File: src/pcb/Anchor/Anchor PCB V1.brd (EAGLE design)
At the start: 100.1 x 68.7 mm, 89 parts, among them IC1 ENC28J60-I_SS, IC2 TPS23750PWP, IC3 MIC5219-3.3YM5-TR, IC4 DWM1000, J1 0826-1X1T-GJ-F, J2 105017-0001, Q1 32 MHz, Q2 SUD06N10-225L, U1 ATSAMD21G-A, Y1 25 MHz

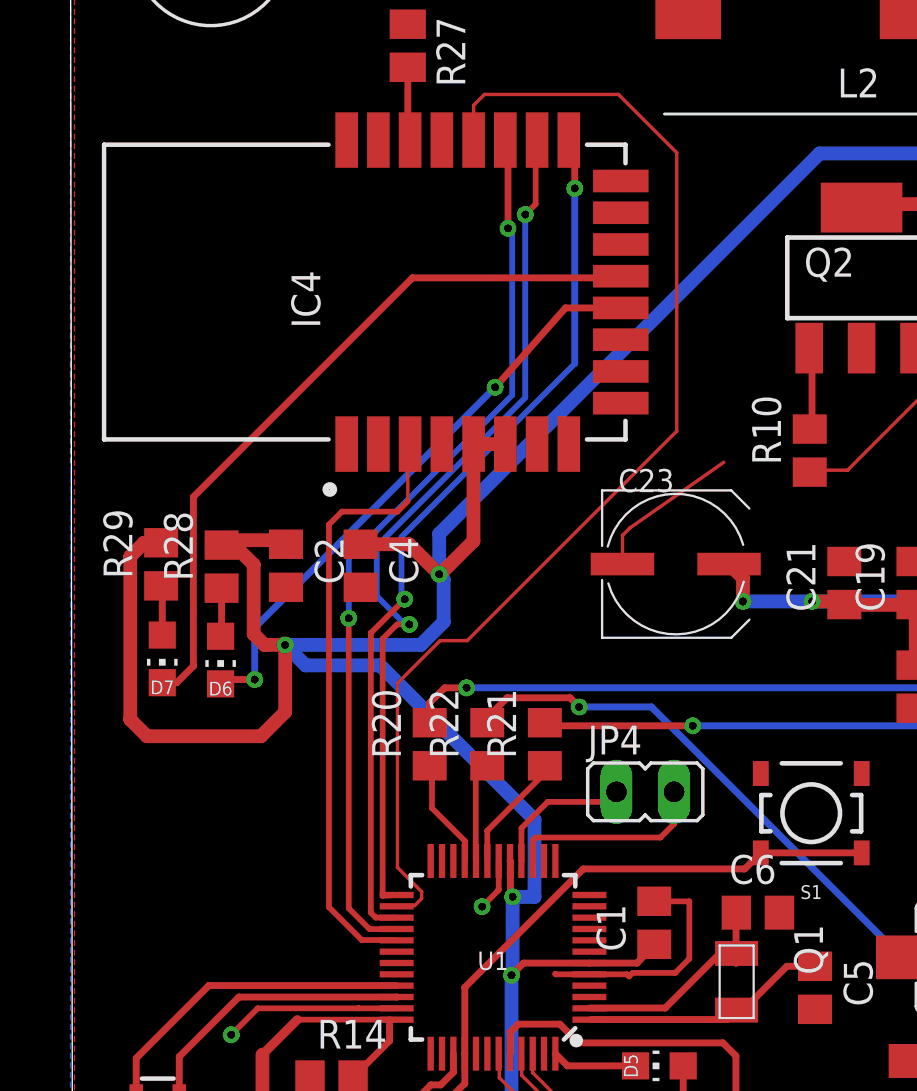
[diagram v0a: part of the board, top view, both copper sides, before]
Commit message: Solving connection problems
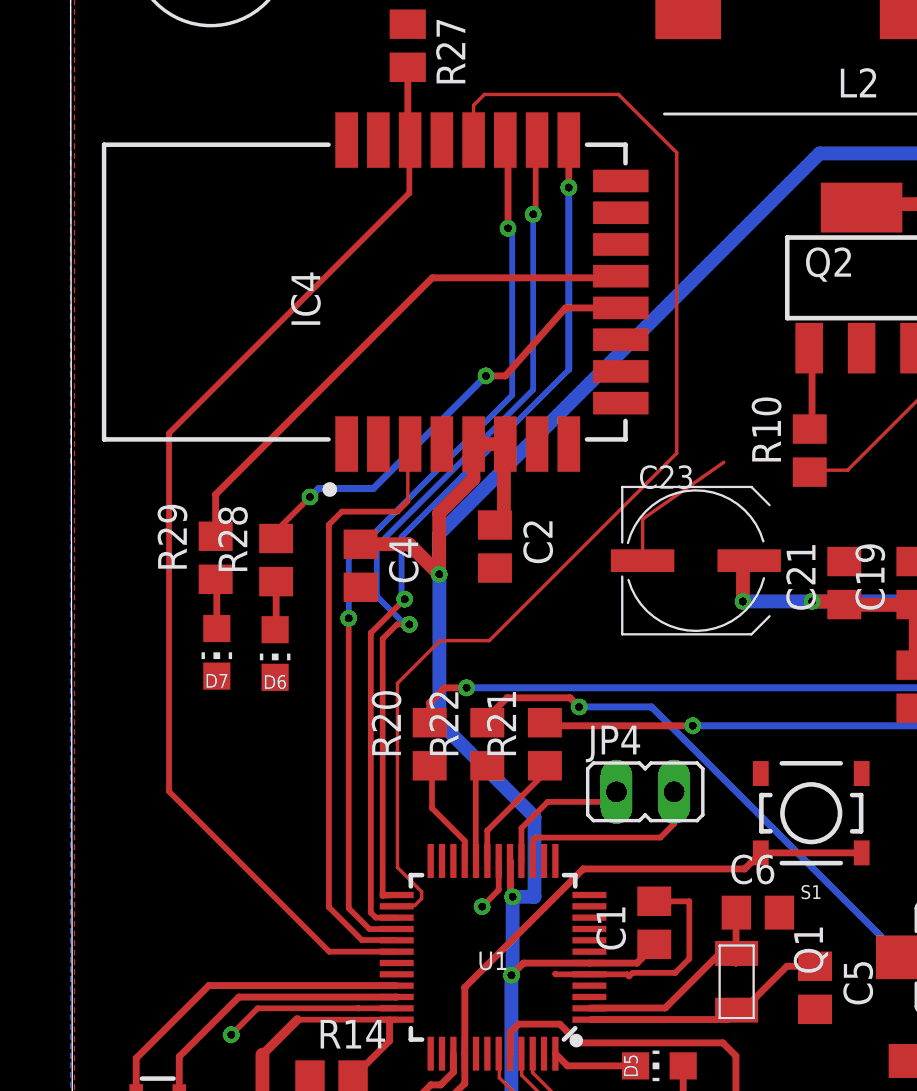
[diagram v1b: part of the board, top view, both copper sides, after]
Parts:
- moved C2 9.25 mm to (18.6, 36.4)
- moved D7 2.42 mm to (6.36, 31.7)
- moved R29 2.42 mm to (6.31, 35.9)
- moved D6 2.42 mm to (8.93, 31.7)
- moved R28 2.42 mm to (8.97, 35.8)
- moved C23 0.90 mm to (27.5, 35.8)
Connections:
- net MISO2_MC renamed MISO2_DWM
- net MOSI2_MC renamed MOSI2_DWM
- net SCK2_MC renamed SCK2_DWM
- net GND: now also D6.C, D7.C
- net IRQ: now also U1.30
- net RXLED_DWM: now also R29.2; no longer D7.C
- net TXLED_DWM: now also R28.2; no longer D6.C
- net VCC: no longer R28.2, R29.2
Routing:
- net IRQ: track 3.25 -> 49.4 mm
- net VCC: track 355.5 -> 319.0 mm, vias 5 -> 4
- net RXLED_DWM: track 32.0 -> 23.7 mm
- net TXLED_DWM: track 26.0 -> 19.9 mm
- net GND: track 49.1 -> 48.5 mm
- net SCK2_DWM: track 52.1 -> 52.7 mm
